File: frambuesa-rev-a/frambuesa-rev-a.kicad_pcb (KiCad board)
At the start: 2 copper layers, 21 x 51 mm, 22 parts, among them J3 Conn_02x18_Odd_Even, J4 Conn_02x18_Odd_Even, U1 RP2040, U2 NCP1117-3.3_SOT223, U3 W25Q128JVS

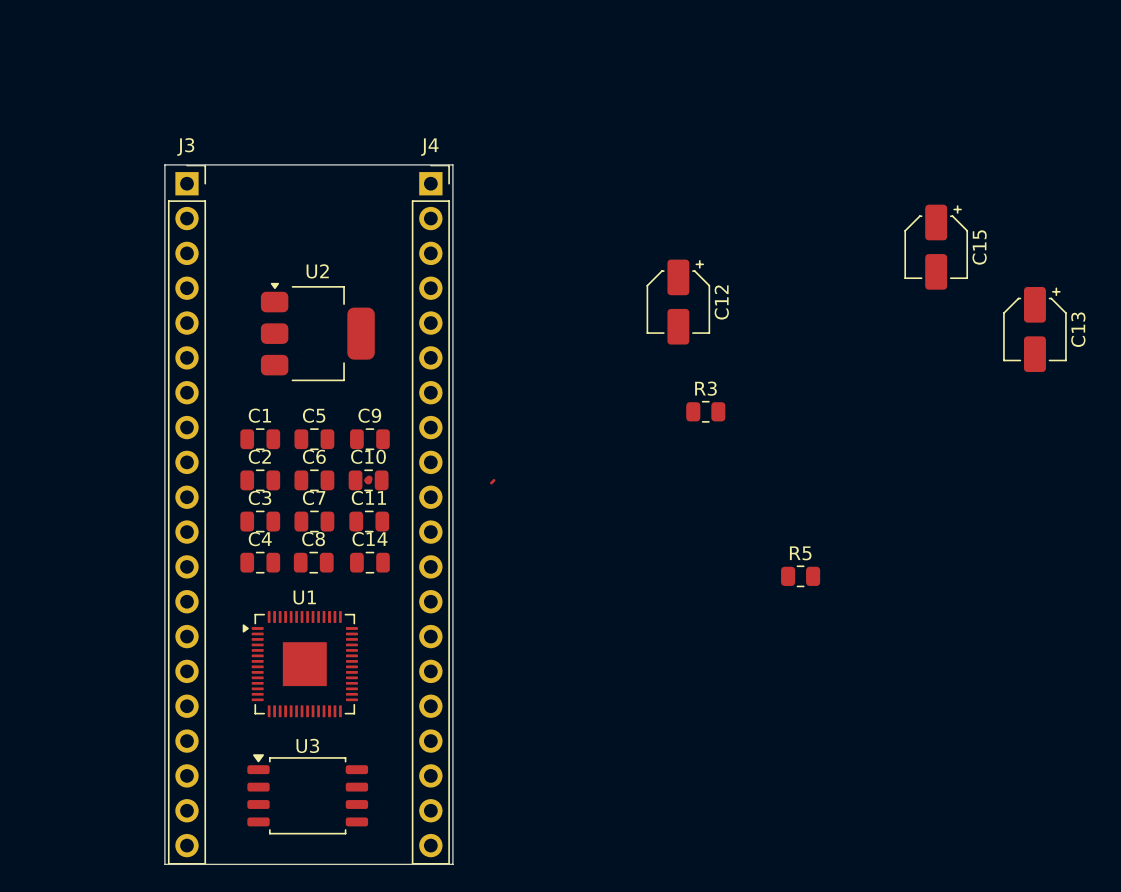
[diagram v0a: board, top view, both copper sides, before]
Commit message: agregar bibliotecas
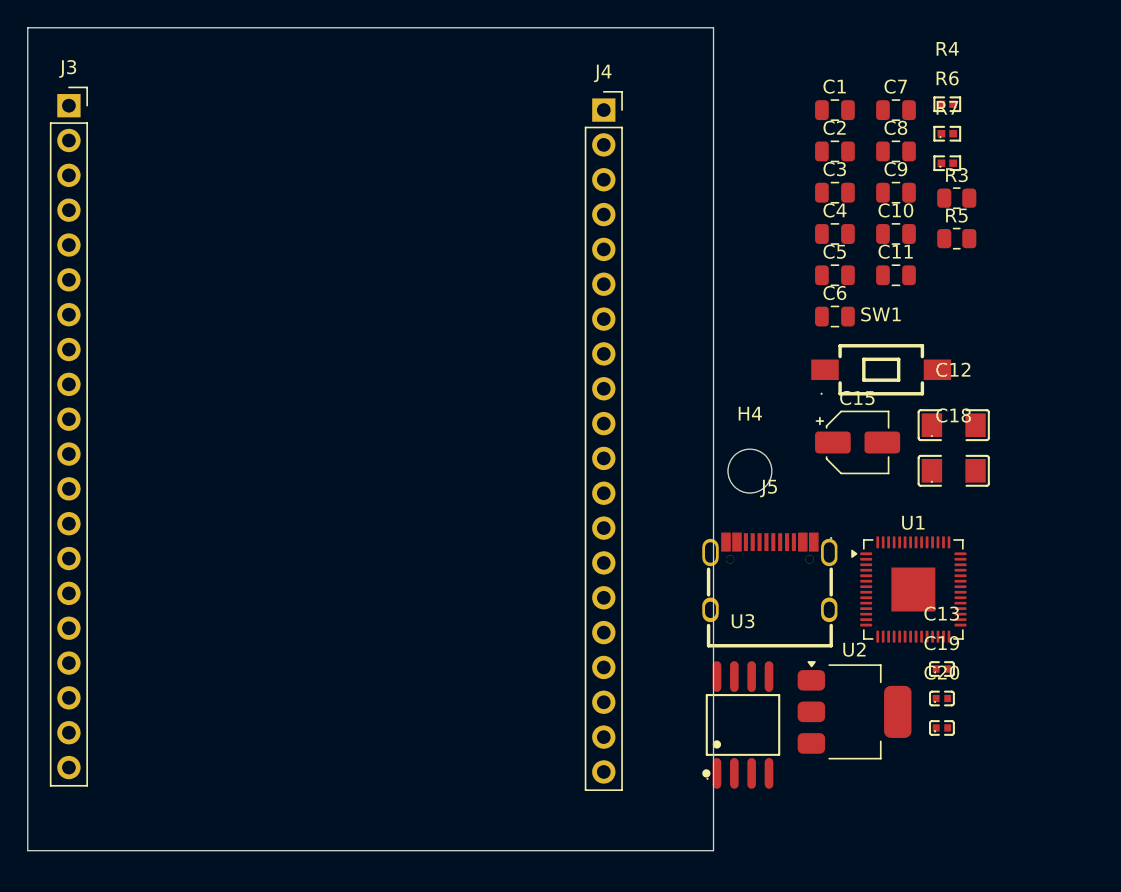
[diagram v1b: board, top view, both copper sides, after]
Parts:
- removed C14: 100n, Capacitor_SMD:C_0805_2012Metric
- added C18: 100u, frambuesa-rev-a:C1206, F.Cu at (87.5, 52.3)
- added C19: 10u, frambuesa-rev-a:C0402, F.Cu at (86.7, 68.9)
- added C20: 10u, frambuesa-rev-a:C0402, F.Cu at (86.7, 71.1)
- added H4: MountingHole, MountingHole:MountingHole_3.2mm_M3, F.Cu at (72.7, 52.3)
- added J5: USB_C_Receptacle_USB2.0_16P, frambuesa-rev-a:USB-C_SMD-TYPE-C-31-M-12_1, F.Cu at (74.1, 60.0)
- added R4: 10k, frambuesa-rev-a:R0402, F.Cu at (87.0, 25.6)
- added R6: 5k1, frambuesa-rev-a:R0402, F.Cu at (87.0, 27.7)
- added R7: 5k1, frambuesa-rev-a:R0402, F.Cu at (87.0, 29.9)
- added SW1: PTS 636, frambuesa-rev-a:KEY-SMD_L6.0-W3.5-LS8.7, F.Cu at (82.2, 44.9)
- C12: value 10u -> 100u; footprint Capacitor_SMD:CP_Elec_4x5.4 -> frambuesa-rev-a:C1206
- C13: footprint Capacitor_SMD:CP_Elec_4x5.4 -> frambuesa-rev-a:C0402
- U2: value NCP1117-3.3_SOT223 -> AMS1117-5.0
- U3: footprint Package_SO:SOIC-8_5.3x5.3mm_P1.27mm -> frambuesa-rev-a:SOIC-8_L5.3-W5.3-P1.27-LS8.0-BL
- moved C8 52.0 mm to (83.3, 29.0)
- moved C7 51.9 mm to (83.3, 26.0)
- moved C1 48.3 mm to (78.9, 26.0)
- moved C2 48.3 mm to (78.9, 29.0)
- moved C3 48.3 mm to (78.9, 32.0)
- moved C4 48.3 mm to (78.9, 35.0)
- moved U2 47.9 mm to (80.3, 69.9)
- moved U1 44.7 mm to (84.6, 61.0)
- moved C10 42.4 mm to (83.3, 35.0)
- moved C11 42.4 mm to (83.3, 38.0)
- moved C9 42.4 mm to (83.3, 32.0)
- moved C5 39.8 mm to (78.9, 38.0)
- moved C6 39.8 mm to (78.9, 41.1)
- moved U3 32.2 mm to (72.2, 70.8)
- moved R5 27.1 mm to (87.7, 35.4)
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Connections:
- C12 pad 1: VBUS -> VHI
- C13 pad 1: +3V3 -> VHI
- R3 pad 2: /NOT_QSPI_SS -> /QSPI_SS
- U2 pad 2: +3V3 -> +3.3V
- U2 pad 3: VBUS -> VHI
- U3 pad 1: /NOT_QSPI_SS -> /QSPI_SS
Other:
- board size 21 x 51 mm -> 50 x 60 mm
